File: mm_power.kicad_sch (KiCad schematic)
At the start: 6 parts, among them J5 Conn_01x02, U3 LP5907MFX-3.3

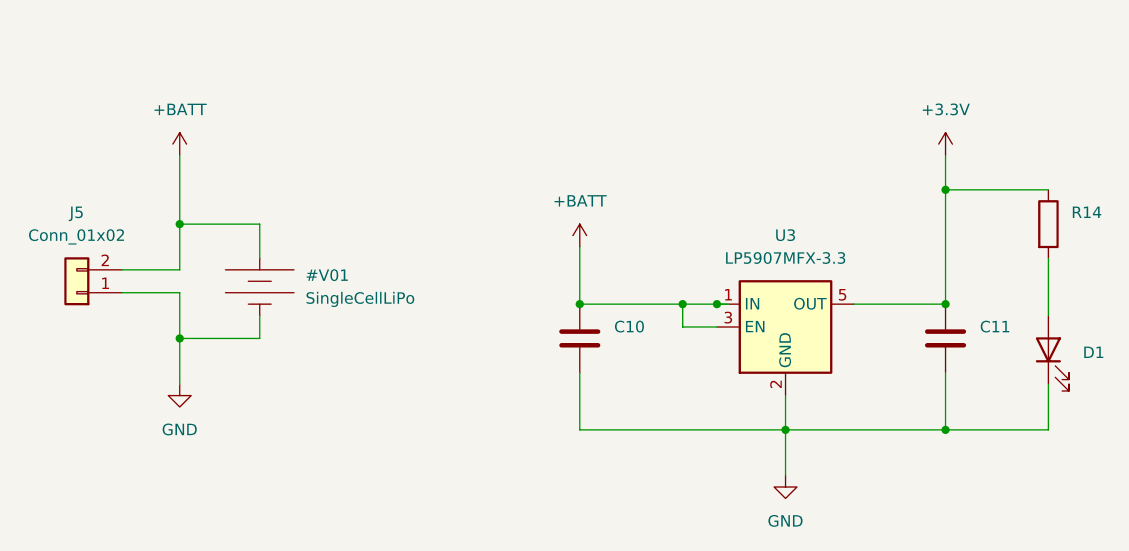
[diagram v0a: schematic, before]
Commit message: heyo
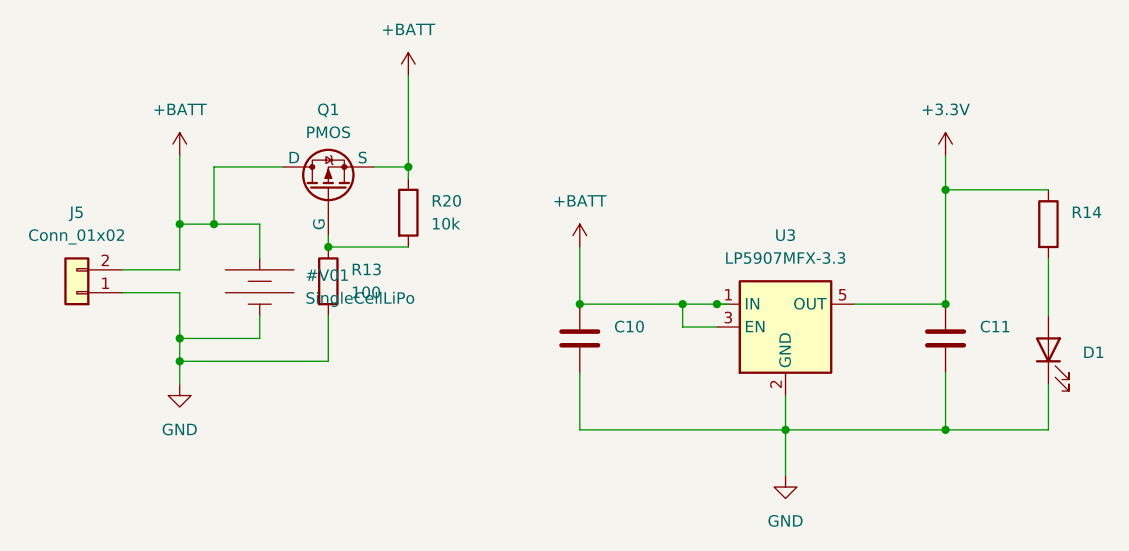
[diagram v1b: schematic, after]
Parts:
- added Q1: PMOS, symbol Simulation_SPICE:PMOS
- added R13: 100, symbol Device:R
- added R20: 10k, symbol Device:R
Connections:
- net +BATT: now also Q1.1 (D), Q1.3 (S), R20.1
- net GND: now also R13.2
- new net: Q1.2 (G), R13.1, R20.2
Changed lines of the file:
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@@
   (junction (at 153.67 105.41) (diameter 0) (color 0 0 0 0)
   )
+  (junction (at 102.87 85.09) (diameter 0) (color 0 0 0 0)
+  )
   (junction (at 171.45 105.41) (diameter 0) (color 0 0 0 0)
   )
@@
   (junction (at 130.81 91.44) (diameter 0) (color 0 0 0 0)
   )
+  (junction (at 111.76 76.2) (diameter 0) (color 0 0 0 0)
+  )
+  (junction (at 90.17 82.55) (diameter 0) (color 0 0 0 0)
+  )
+  (junction (at 86.36 97.79) (diameter 0) (color 0 0 0 0)
+  )
   (junction (at 142.24 91.44) (diameter 0) (color 0 0 0 0)
   )
@@
     (stroke (width 0) (type default))
   )
+  (wire (pts (xy 102.87 97.79) (xy 86.36 97.79))
+    (stroke (width 0) (type default))
+  )
   (wire (pts (xy 182.88 86.36) (xy 182.88 92.71))
     (stroke (width 0) (type default))
@@
     (stroke (width 0) (type default))
   )
-  (wire (pts (xy 95.25 82.55) (xy 86.36 82.55))
+  (wire (pts (xy 90.17 82.55) (xy 86.36 82.55))
+    (stroke (width 0) (type default))
+  )
+  (wire (pts (xy 111.76 66.04) (xy 111.76 76.2))
+    (stroke (width 0) (type default))
+  )
+  (wire (pts (xy 102.87 85.09) (xy 111.76 85.09))
+    (stroke (width 0) (type default))
+  )
+  (wire (pts (xy 95.25 82.55) (xy 90.17 82.55))
     (stroke (width 0) (type default))
   )
@@
     (stroke (width 0) (type default))
   )
+  (wire (pts (xy 102.87 92.71) (xy 102.87 97.79))
+    (stroke (width 0) (type default))
+  )
+  (wire (pts (xy 86.36 97.79) (xy 86.36 100.33))
+    (stroke (width 0) (type default))
+  )
   (wire (pts (xy 130.81 105.41) (xy 153.67 105.41))
     (stroke (width 0) (type default))
@@
     (stroke (width 0) (type default))
   )
+  (wire (pts (xy 111.76 76.2) (xy 111.76 77.47))
+    (stroke (width 0) (type default))
+  )
   (wire (pts (xy 130.81 91.44) (xy 142.24 91.44))
     (stroke (width 0) (type default))
@@
     (stroke (width 0) (type default))
   )
-  (wire (pts (xy 86.36 95.25) (xy 86.36 100.33))
+  (wire (pts (xy 86.36 95.25) (xy 86.36 97.79))
     (stroke (width 0) (type default))
   )
@@
     (stroke (width 0) (type default))
   )
+  (wire (pts (xy 97.79 76.2) (xy 90.17 76.2))
+    (stroke (width 0) (type default))
+  )
   (wire (pts (xy 182.88 105.41) (xy 171.45 105.41))
     (stroke (width 0) (type default))
@@
     (stroke (width 0) (type default))
   )
+  (wire (pts (xy 102.87 83.82) (xy 102.87 85.09))
+    (stroke (width 0) (type default))
+  )
   (wire (pts (xy 142.24 93.98) (xy 142.24 91.44))
     (stroke (width 0) (type default))
   )
+  (wire (pts (xy 111.76 76.2) (xy 107.95 76.2))
+    (stroke (width 0) (type default))
+  )
   (wire (pts (xy 171.45 74.93) (xy 171.45 78.74))
     (stroke (width 0) (type default))
@@
   )
   (wire (pts (xy 161.29 91.44) (xy 171.45 91.44))
+    (stroke (width 0) (type default))
+  )
+  (wire (pts (xy 90.17 76.2) (xy 90.17 82.55))
     (stroke (width 0) (type default))
   )
@@
     )
   )
+  (symbol (lib_id "Simulation_SPICE:PMOS") (at 102.87 78.74 90) (unit 1)
+    (in_bom yes) (on_board yes) (dnp no) (fields_autoplaced)
+    (property "Reference" "Q1" (at 102.87 69.85 90)
+      (effects (font (size 1.27 1.27)))
+    )
+    (property "Value" "PMOS" (at 102.87 72.39 90)
+      (effects (font (size 1.27 1.27)))
+    )
+    (property "Footprint" "" (at 100.33 73.66 0)
+      (effects (font (size 1.27 1.27)) hide)
+    )
+    (property "Datasheet" "https://ngspice.sourceforge.io/docs/ngspice-manual.pdf" (at 115.57 78.74 0)
+      (effects (font (size 1.27 1.27)) hide)
+    )
+    (property "Sim.Device" "PMOS" (at 120.015 78.74 0)
+      (effects (font (size 1.27 1.27)) hide)
+    )
+    (property "Sim.Type" "VDMOS" (at 121.92 78.74 0)
+      (effects (font (size 1.27 1.27)) hide)
+    )
+    (property "Sim.Pins" "1=D 2=G 3=S" (at 118.11 78.74 0)
+      (effects (font (size 1.27 1.27)) hide)
+    )
+    (pin "2")
+    (pin "1")
+    (pin "3")
+    (instances
+      (project "minimouse"
+        (path "/d8fa4cba-2469-4231-847f-065b6b829f44/3f9b0845-5778-418c-a7a8-03da2392145e"
+          (reference "Q1") (unit 1)
+        )
+      )
+    )
+  )
   (symbol (lib_id "Regulator_Linear:LP5907MFX-3.3") (at 153.67 93.98 0) (unit 1)
     (in_bom yes) (on_board yes) (dnp no) (fields_autoplaced)
@@
         )
       )
+    )
+  )
+  (symbol (lib_id "Device:R") (at 111.76 81.28 0) (unit 1)
+    (in_bom yes) (on_board yes) (dnp no) (fields_autoplaced)
+    (property "Reference" "R20" (at 114.3 80.01 0)
+      (effects (font (size 1.27 1.27)) (justify left))
+    )
+    (property "Value" "10k" (at 114.3 82.55 0)
+      (effects (font (size 1.27 1.27)) (justify left))
+    )
+    (property "Footprint" "" (at 109.982 81.28 90)
+      (effects (font (size 1.27 1.27)) hide)
+    )
+    (property "Datasheet" "~" (at 111.76 81.28 0)
+      (effects (font (size 1.27 1.27)) hide)
+    )
+    (pin "2")
+    (pin "1")
+    (instances
+      (project "minimouse"
+        (path "/d8fa4cba-2469-4231-847f-065b6b829f44/3f9b0845-5778-418c-a7a8-03da2392145e"
+          (reference "R20") (unit 1)
+        )
+      )
+    )
+  )
+  (symbol (lib_id "Device:R") (at 102.87 88.9 0) (unit 1)
+    (in_bom yes) (on_board yes) (dnp no) (fields_autoplaced)
+    (property "Reference" "R13" (at 105.41 87.63 0)
+      (effects (font (size 1.27 1.27)) (justify left))
+    )
+    (property "Value" "100" (at 105.41 90.17 0)
+      (effects (font (size 1.27 1.27)) (justify left))
+    )
+    (property "Footprint" "" (at 101.092 88.9 90)
+      (effects (font (size 1.27 1.27)) hide)
+    )
+    (property "Datasheet" "~" (at 102.87 88.9 0)
+      (effects (font (size 1.27 1.27)) hide)
+    )
+    (pin "1")
+    (pin "2")
+    (instances
+      (project "minimouse"
+        (path "/d8fa4cba-2469-4231-847f-065b6b829f44/3f9b0845-5778-418c-a7a8-03da2392145e"
+          (reference "R13") (unit 1)
+        )
+      )
+    )
+  )
+  (symbol (lib_id "power:+BATT") (at 111.76 66.04 0) (unit 1)
+    (in_bom yes) (on_board yes) (dnp no) (fields_autoplaced)
+    (property "Reference" "#PWR027" (at 111.76 69.85 0)
+      (effects (font (size 1.27 1.27)) hide)
+    )
+    (property "Value" "+BATT" (at 111.76 60.96 0)
+      (effects (font (size 1.27 1.27)))
+    )
+    (property "Footprint" "" (at 111.76 66.04 0)
+      (effects (font (size 1.27 1.27)) hide)
+    )
+    (property "Datasheet" "" (at 111.76 66.04 0)
+      (effects (font (size 1.27 1.27)) hide)
+    )
+    (pin "1")
+    (instances
+      (project "minimouse"
+        (path "/d8fa4cba-2469-4231-847f-065b6b829f44/3f9b0845-5778-418c-a7a8-03da2392145e"
+          (reference "#PWR027") (unit 1)
+        )
+      )
